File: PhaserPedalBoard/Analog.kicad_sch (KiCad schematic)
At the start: 63 parts, among them Q4 BC847, Q5 BC857, Q6 BC857, SW1 COLOR, U2 LM13700, U3 LM13700, U5 TL074

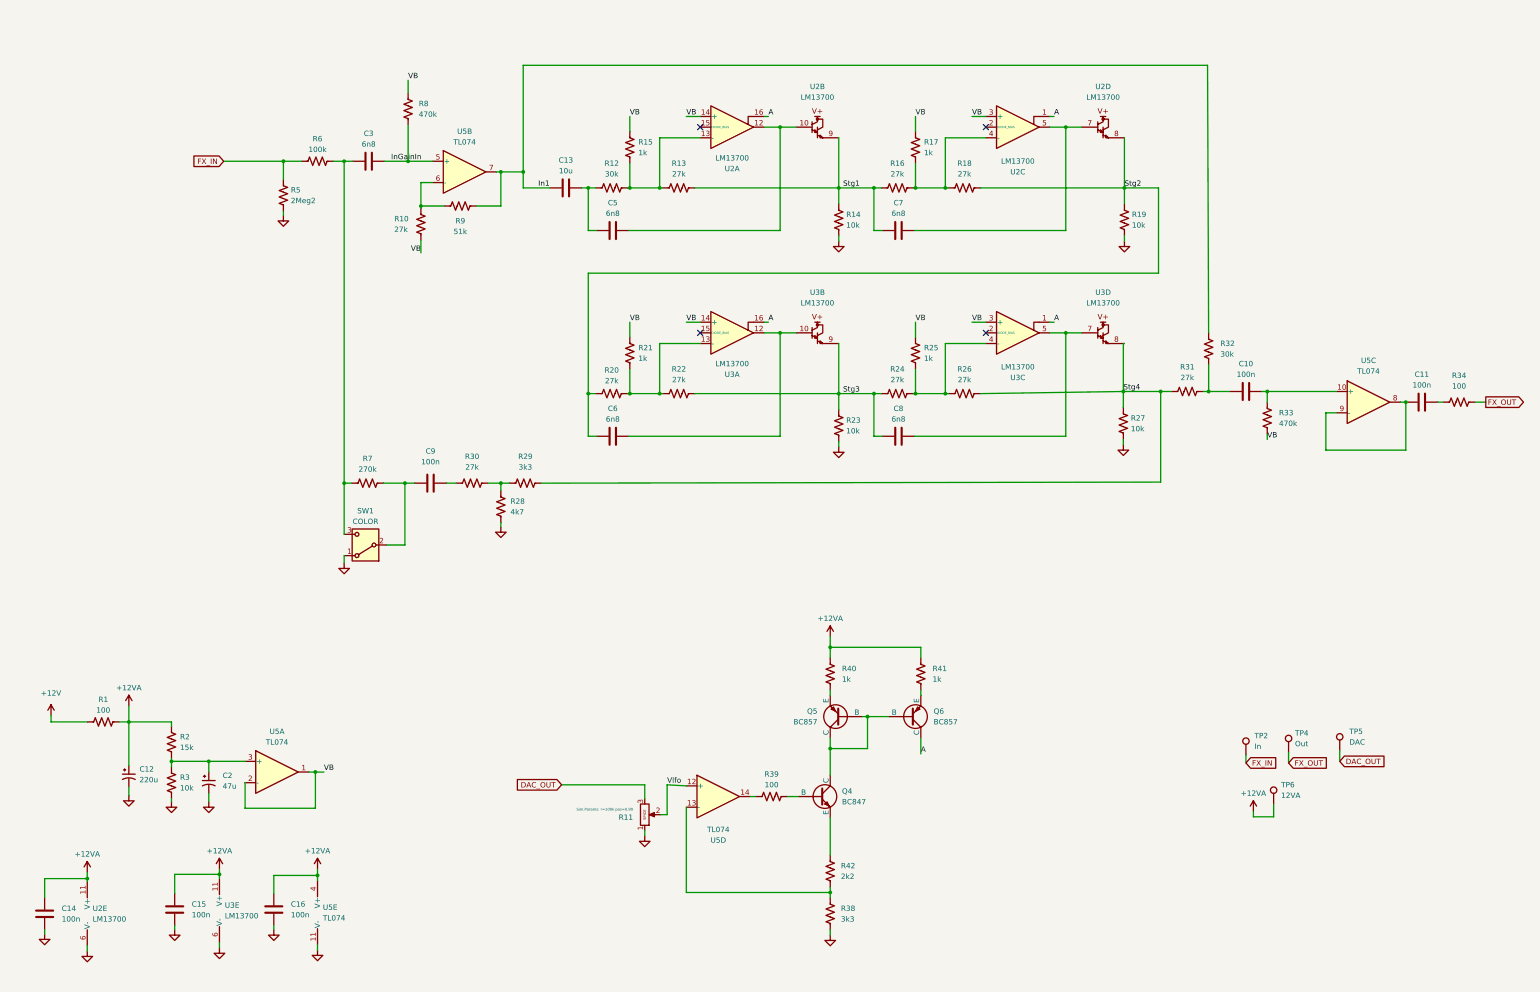
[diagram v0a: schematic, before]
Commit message: schematic hygiene
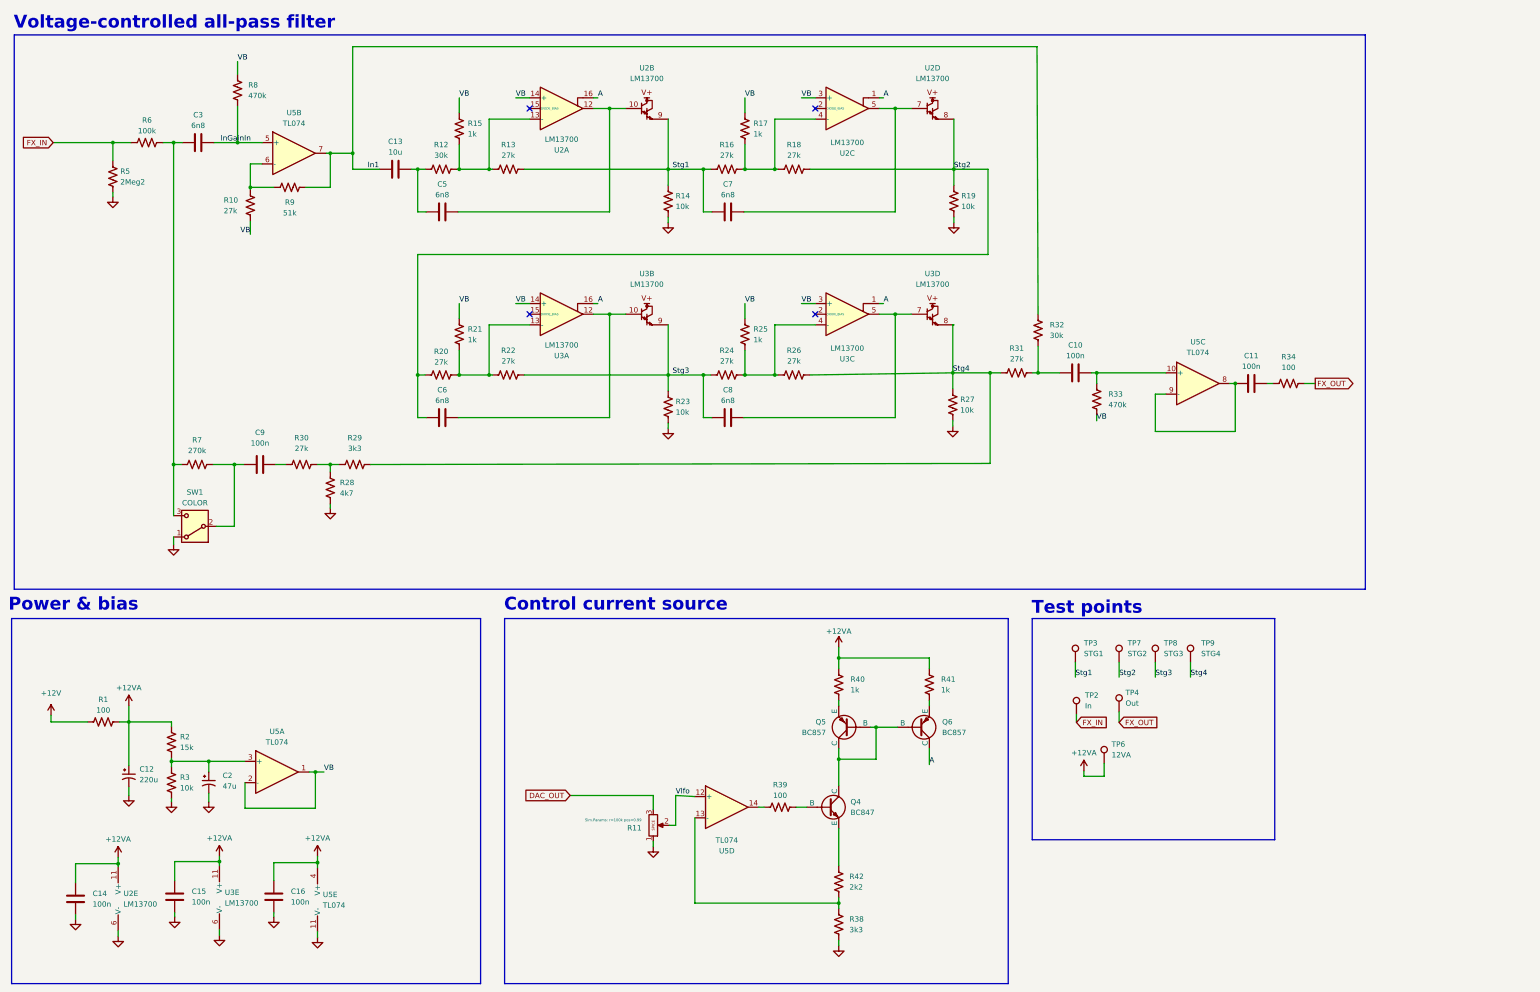
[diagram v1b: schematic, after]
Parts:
- removed TP5: DAC, TestPoint:TestPoint_THTPad_D2.0mm_Drill1.0mm_VAL, symbol Connector:TestPoint
- added TP3: STG1, TestPoint:TestPoint_THTPad_D2.0mm_Drill1.0mm_VAL, symbol Connector:TestPoint
- added TP7: STG2, TestPoint:TestPoint_THTPad_D2.0mm_Drill1.0mm_VAL, symbol Connector:TestPoint
- added TP8: STG3, TestPoint:TestPoint_THTPad_D2.0mm_Drill1.0mm_VAL, symbol Connector:TestPoint
- added TP9: STG4, TestPoint:TestPoint_THTPad_D2.0mm_Drill1.0mm_VAL, symbol Connector:TestPoint
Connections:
- net Stg1: now also TP3.1
- net Stg2: now also TP7.1
- net Stg3: now also TP8.1
- net Stg4: now also TP9.1
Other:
- note added: "Control current source"
- note added: "Power & bias"
- note added: "Test points"
- note added: "Voltage-controlled all-pass filter"
- moved on the sheet: C10, C11, C13, C14, C15, C16, C3, C5, C6, C7, C8, C9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

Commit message: rough layout
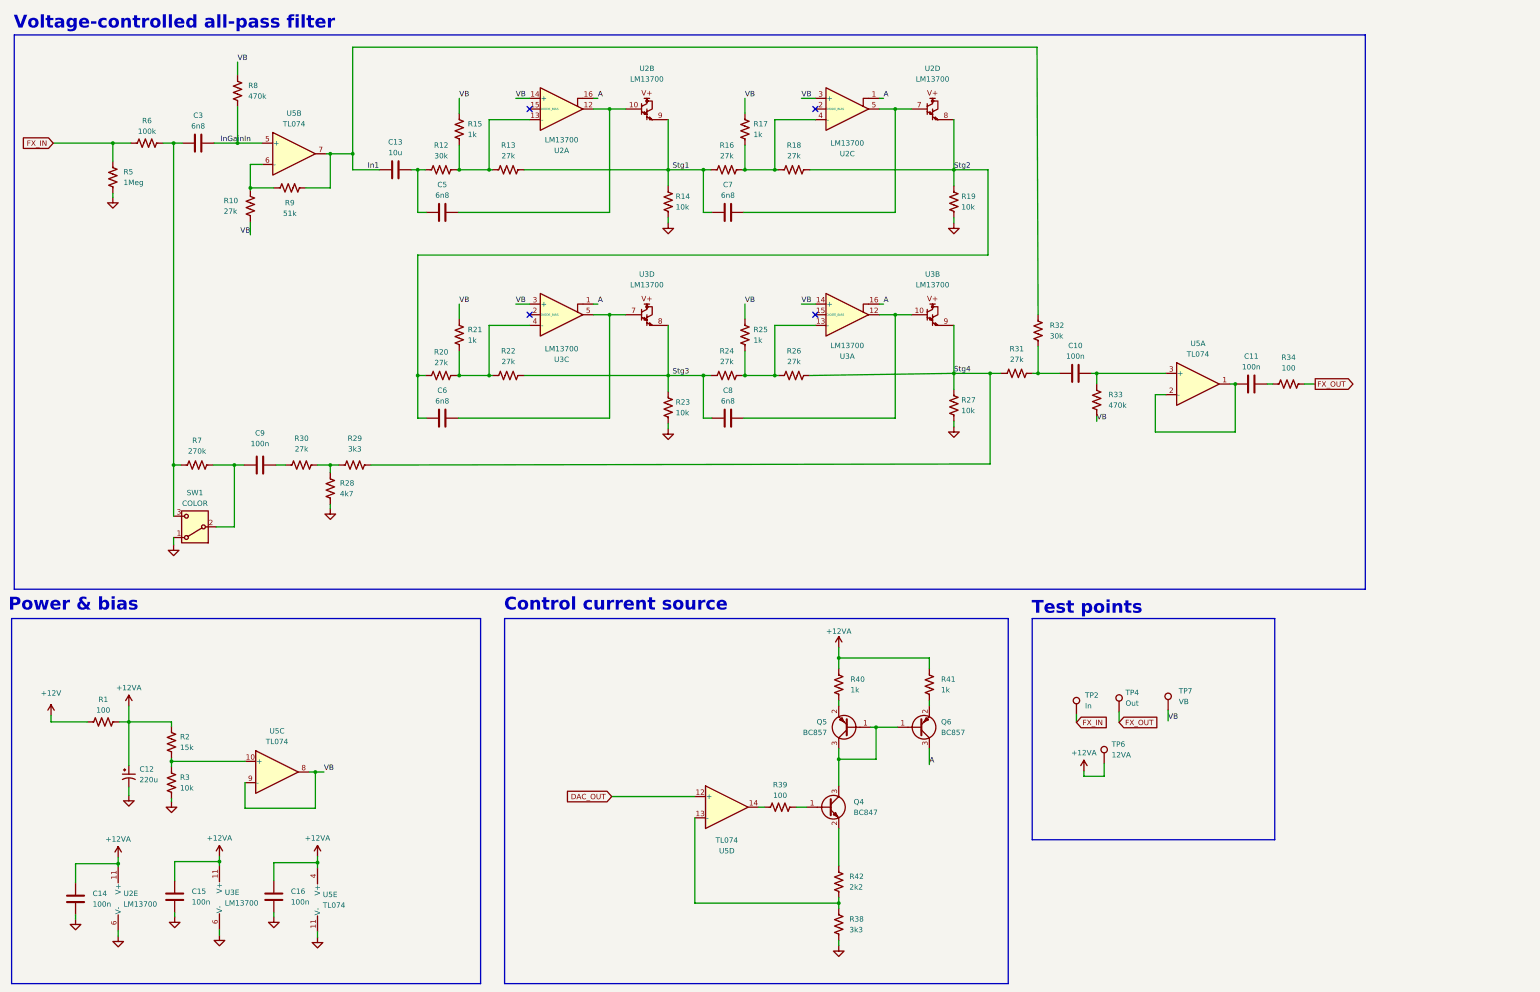
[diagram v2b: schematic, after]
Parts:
- removed C2: 47u, symbol Device:C_Polarized_Small_US
- removed Q4: BC847, symbol Simulation_SPICE:NPN
- removed Q5, Q6: BC857, symbol Simulation_SPICE:PNP
- removed R11: Potentiometer, symbol Simulation_SPICE:Potentiometer
- removed TP3: STG1, TestPoint:TestPoint_THTPad_D2.0mm_Drill1.0mm_VAL, symbol Connector:TestPoint
- removed TP8: STG3, TestPoint:TestPoint_THTPad_D2.0mm_Drill1.0mm_VAL, symbol Connector:TestPoint
- removed TP9: STG4, TestPoint:TestPoint_THTPad_D2.0mm_Drill1.0mm_VAL, symbol Connector:TestPoint
- added Q4: BC847, Package_TO_SOT_SMD:SOT-23, symbol Transistor_BJT:BC847
- added Q5, Q6: BC857, Package_TO_SOT_SMD:SOT-23, symbol Transistor_BJT:BC857
- C10, C11, C13, C14, C15, C16, C3, C5, C6, C7, C8, C9: footprint (none) -> Capacitor_SMD:C_0805_2012Metric
- C12: footprint (none) -> Capacitor_THT:CP_Radial_D7.5mm_P2.50mm
- R1, R10, R12, R13, R14, R15, R16, R17, R18, R19, R2, R20, R21, R22, R23, R24, R25, R26, R27, R28, R29, R3, R30, R31, R32, R33, R34, R38, R39, R40, R41, R42, R6, R7, R8, R9: footprint (none) -> Resistor_SMD:R_0805_2012Metric
- R5: value 2Meg2 -> 1Meg; footprint (none) -> Resistor_SMD:R_0805_2012Metric
- TP7: value STG2 -> VB
- U2, U3: footprint (none) -> Package_SO:SOIC-16_3.9x9.9mm_P1.27mm
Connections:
- net Vlfo is gone; now on net DAC_OUT: U5.12 (+)
- net A: now also Q6.3 (C)
- net Stg2: no longer TP7.1
- net Stg3: now also U3.8; no longer U3.9
- net Stg4: now also U3.9; no longer U3.8
- net VB: now also TP7.1, U5.8, U5.9 (-); no longer U5.1, U5.2 (-)
- net at U3.5, U3.7: now also C6.2; no longer C8.2
- net at R20.1, R21.2, R22.2: now also U3.4 (-); no longer U3.13 (-)
- net at C10.2, R33.1: now also U5.3 (+); no longer U5.10 (+)
- net at R24.1, R25.2, R26.2: now also U3.13 (-); no longer U3.4 (-)
- net at R2.1, R3.2: now also U5.10 (+); no longer U5.3 (+)
- net at U3.10, U3.12: now also C8.2; no longer C6.2
- net at R41.1: now also Q6.2 (E)
- net at R39.2: now also Q4.1 (B)
- net at R42.2: now also Q4.2 (E)
- net at R40.1: now also Q5.2 (E)
- new net: C11.1, U5.1, U5.2 (-)
- new net: Q4.3 (C), Q5.1 (B), Q5.3 (C), Q6.1 (B)
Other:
- moved on the sheet: U3A, U3B, U3C, U3D, U5A, U5C
